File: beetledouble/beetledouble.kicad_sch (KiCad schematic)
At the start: 28 parts, among them J1 XT30PW-M, J2 rxin, J6 prog connector, U1 78L12G-AB3-R, U2 DD4012SB, U3 ATtiny1614-SS

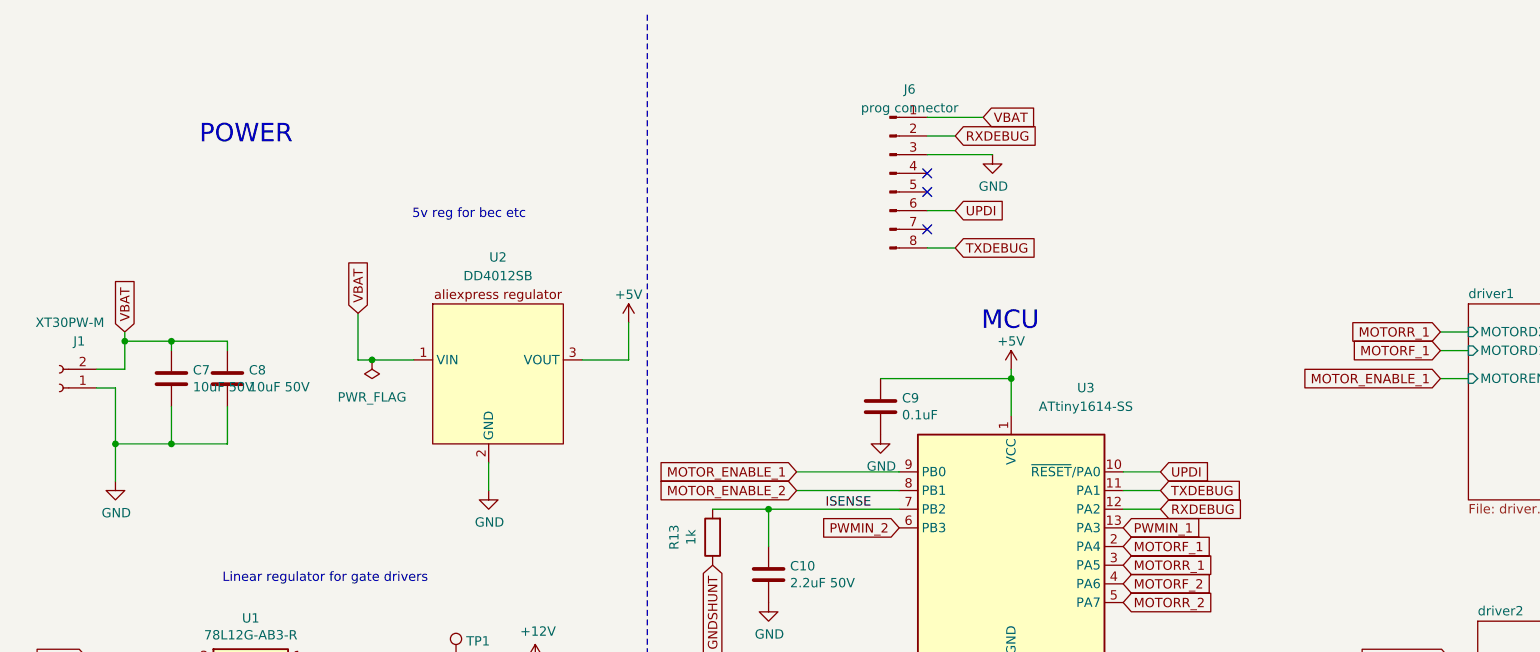
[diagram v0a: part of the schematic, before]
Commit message: Updates
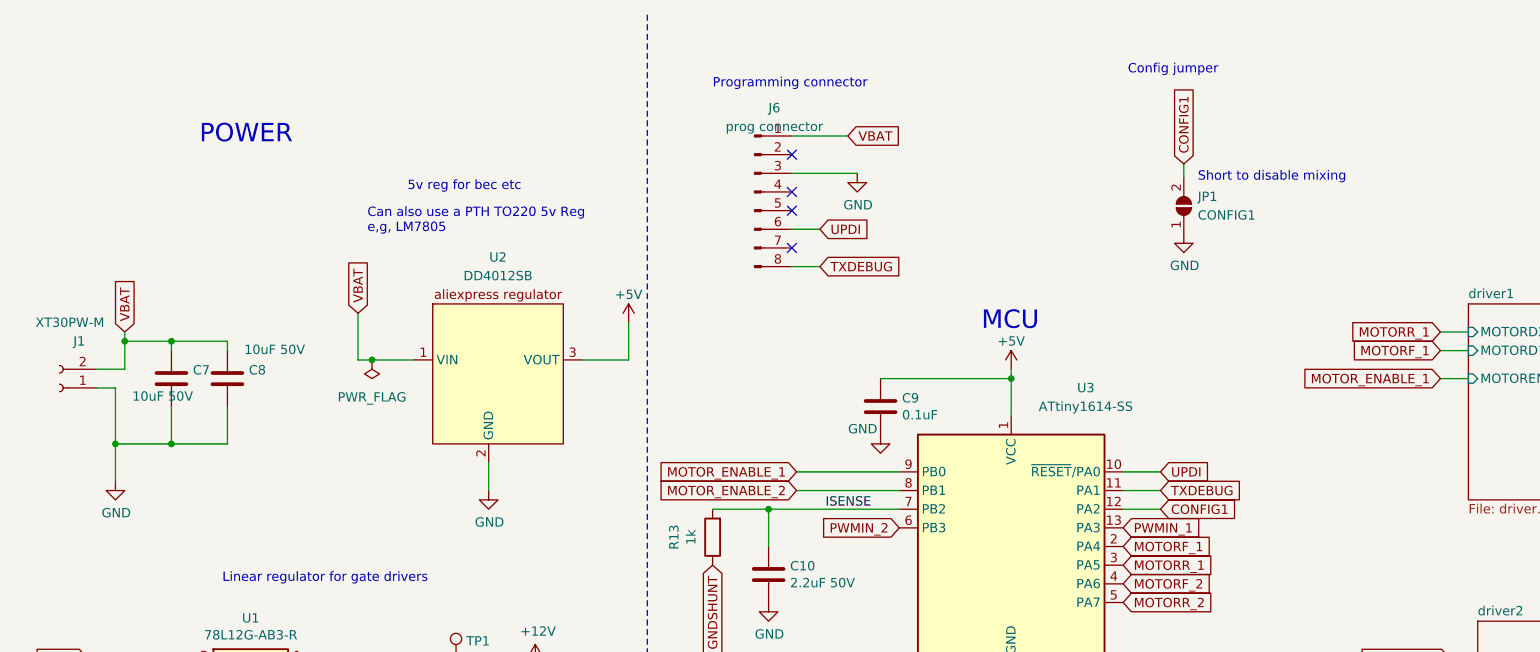
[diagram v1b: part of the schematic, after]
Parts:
- added JP1: CONFIG1, Jumper:SolderJumper-2_P1.3mm_Open_TrianglePad1.0x1.5mm, symbol Jumper:SolderJumper_2_Open
- C10, C2: LCSC C326557 -> C162273
- R10, R13, R14, R15, R9: LCSC (none) -> C21190
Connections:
- net GND: now also JP1.1 (A)
- net RXDEBUG: no longer names the net of J6.2 (Pin_2)
- net RXDEBUG: no longer U3.12 (PA2)
- new net CONFIG1: JP1.2 (B), U3.12 (PA2)
- no-connect marks 5 -> 6
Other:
- note added: "Can also use a PTH TO220 5v Reg e,g, LM7805"
- note added: "Config jumper"
- note added: "Programming connector"
- note added: "Short to disable mixing"
- moved on the sheet: J6

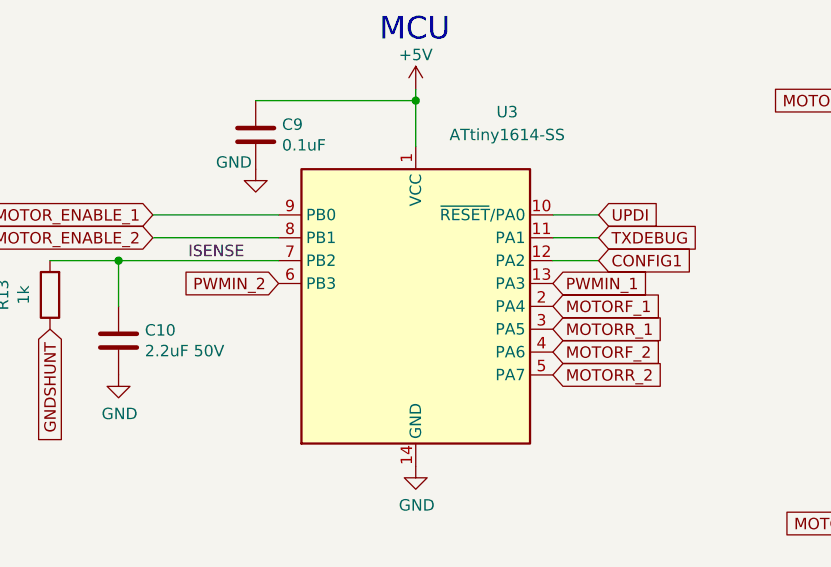
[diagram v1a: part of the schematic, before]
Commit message: Updates
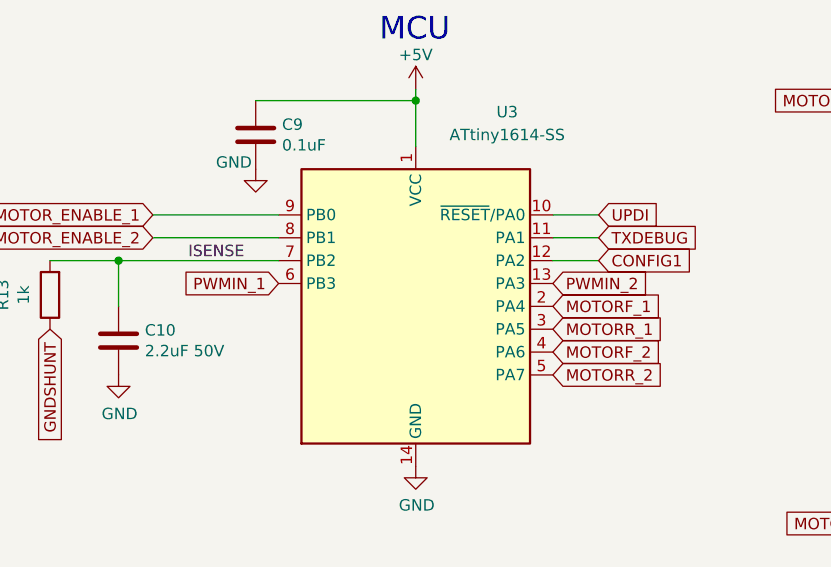
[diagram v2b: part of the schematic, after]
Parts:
- R11, R12: LCSC (none) -> C146895
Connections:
- net PWMIN_1: now also U3.6 (PB3); no longer U3.13 (PA3)
- net PWMIN_2: now also U3.13 (PA3); no longer U3.6 (PB3)
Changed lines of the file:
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@@
     )
   )
-  (global_label "PWMIN_2" (shape input) (at 137.16 81.28 180) (fields_autoplaced)
+  (global_label "PWMIN_1" (shape input) (at 137.16 81.28 180) (fields_autoplaced)
     (effects (font (size 1.27 1.27)) (justify right))
     (property "Intersheet References" "${INTERSHEET_REFS}" (id 0) (at 126.4617 81.3594 0)
@@
     )
   )
-  (global_label "PWMIN_1" (shape input) (at 167.64 81.28 0) (fields_autoplaced)
+  (global_label "PWMIN_2" (shape input) (at 167.64 81.28 0) (fields_autoplaced)
     (effects (font (size 1.27 1.27)) (justify left))
     (property "Intersheet References" "${INTERSHEET_REFS}" (id 0) (at 178.3383 81.2006 0)
@@
       (effects (font (size 1.27 1.27)) hide)
     )
+    (property "LCSC" "C146895" (id 4) (at 195.58 143.51 0)
+      (effects (font (size 1.27 1.27)) hide)
+    )
     (pin "1")
     (pin "2")
@@
       (effects (font (size 1.27 1.27)) hide)
     )
+    (property "LCSC" "C146895" (id 4) (at 210.185 143.51 0)
+      (effects (font (size 1.27 1.27)) hide)
+    )
